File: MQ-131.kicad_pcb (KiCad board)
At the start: 2 copper layers, 26.5 x 64 mm, 11 parts, among them J1 Conn_01x04_Pin

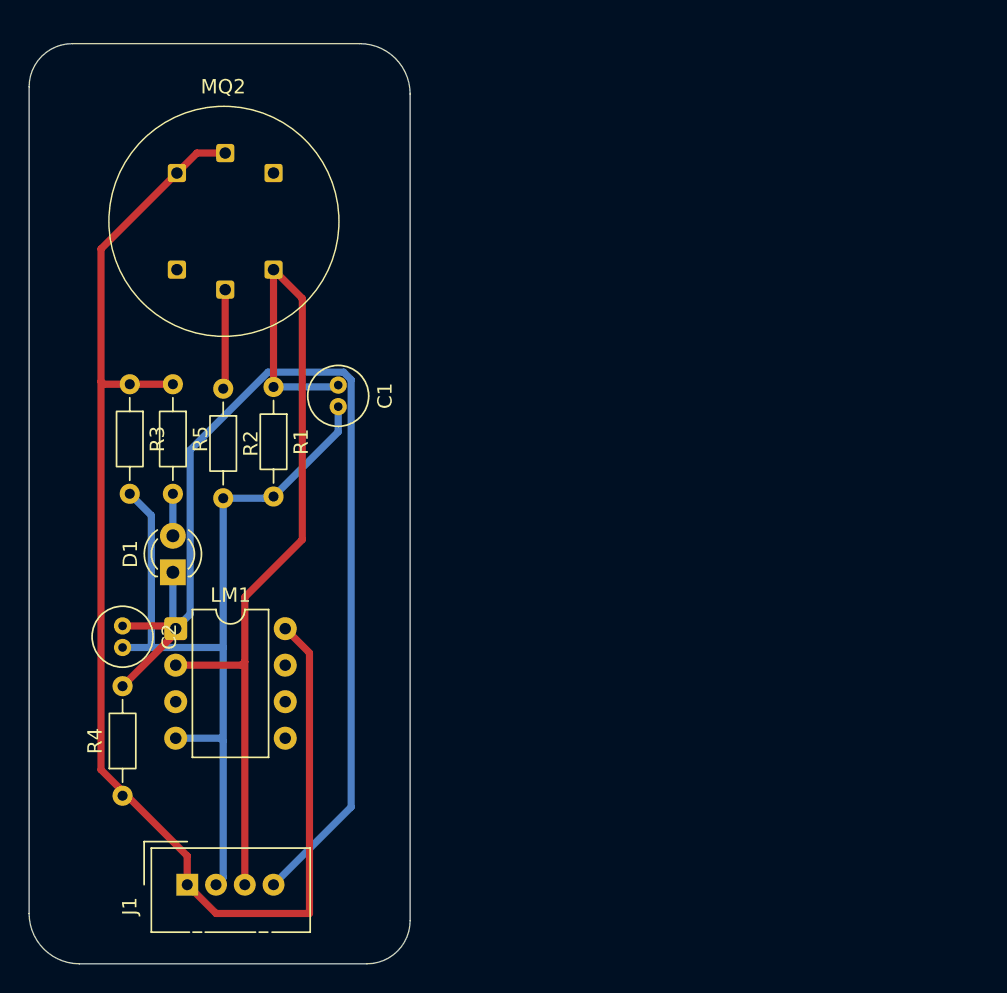
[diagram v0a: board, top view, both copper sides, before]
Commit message: PCB board design altered
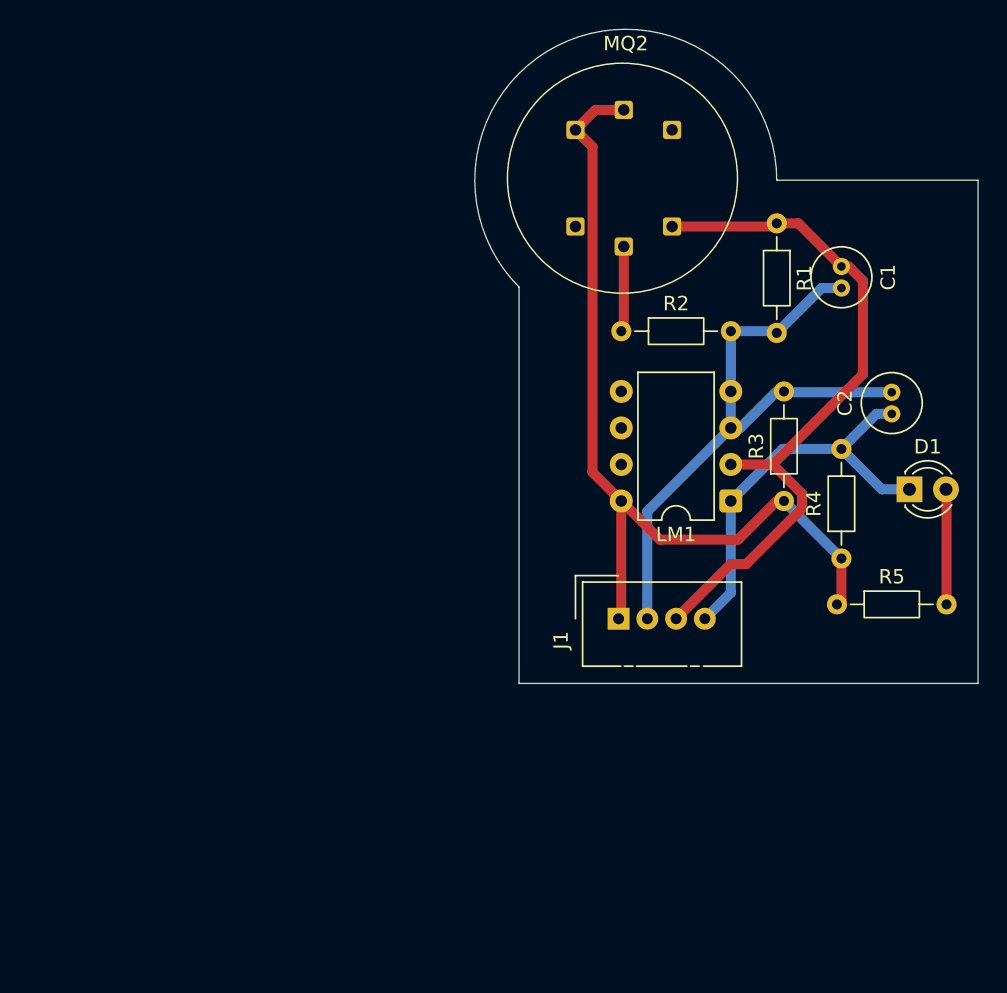
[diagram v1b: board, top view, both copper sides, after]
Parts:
- moved C2 55.5 mm to (240.5, 80.2), turned to 90 degrees
- moved R4 52.7 mm to (237.0, 90.3)
- moved D1 51.6 mm to (241.7, 85.5), turned to 0 degrees
- moved R5 48.7 mm to (236.7, 93.5), turned to 0 degrees
- moved R3 46.2 mm to (233.0, 86.3), turned to 90 degrees
- moved LM1 39.6 mm to (229.3, 86.3), turned to 180 degrees
- moved R1 36.8 mm to (232.5, 67.0)
- moved C1 36.0 mm to (237.0, 70.0)
- moved J1 35.2 mm to (221.5, 94.5)
- moved R2 28.0 mm to (221.7, 74.5), turned to 0 degrees
- moved MQ2 27.9 mm to (221.9, 63.9)
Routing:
- net /DOUT: track 77.2 -> 28.5 mm, vias 0 -> 1
- net VCC: track 93.0 -> 61.4 mm
- net GND: track 60.4 -> 43.2 mm
- net /AOUT: track 63.1 -> 49.1 mm
- net Net-(D1-A): track 2.92 -> 8.02 mm
- net Net-(MQ2-H2): track 6.95 -> 5.96 mm
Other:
- board size 26.5 x 64 mm -> 35 x 45.5 mm
